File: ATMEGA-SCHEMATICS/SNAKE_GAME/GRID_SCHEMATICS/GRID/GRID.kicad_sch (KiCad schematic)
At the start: 400 parts, among them J1 Conn_01x04_Pin, J2 Conn_01x04_Pin

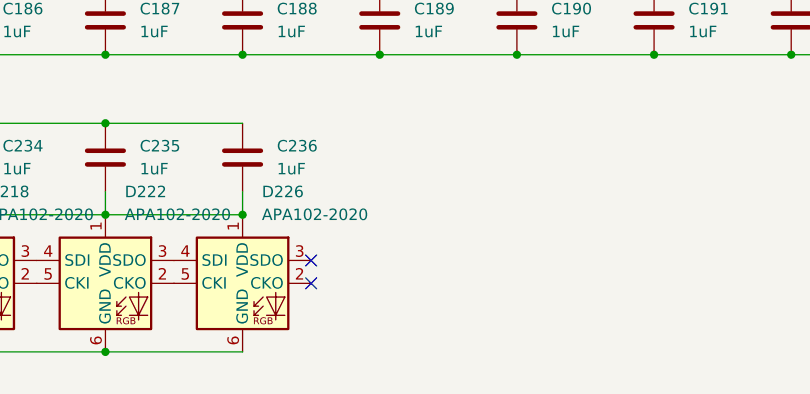
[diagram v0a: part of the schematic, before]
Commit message: .
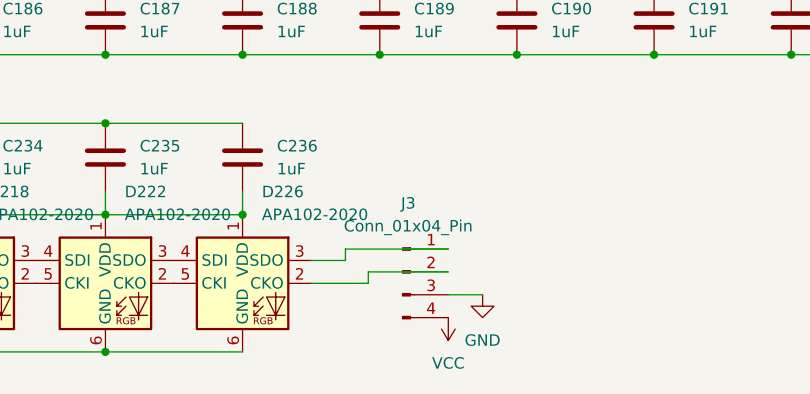
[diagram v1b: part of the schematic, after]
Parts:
- added J3: Conn_01x04_Pin, Connector_PinHeader_2.54mm:PinHeader_1x04_P2.54mm_Vertical, symbol Connector:Conn_01x04_Pin
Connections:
- net GND: now also J3.3 (Pin_3)
- net VCC: now also J3.4 (Pin_4)
- net at D226.2 (CKO): now also J3.2 (Pin_2)
- net at D226.3 (SDO): now also J3.1 (Pin_1)
- no-connect marks 2 -> 0

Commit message: .
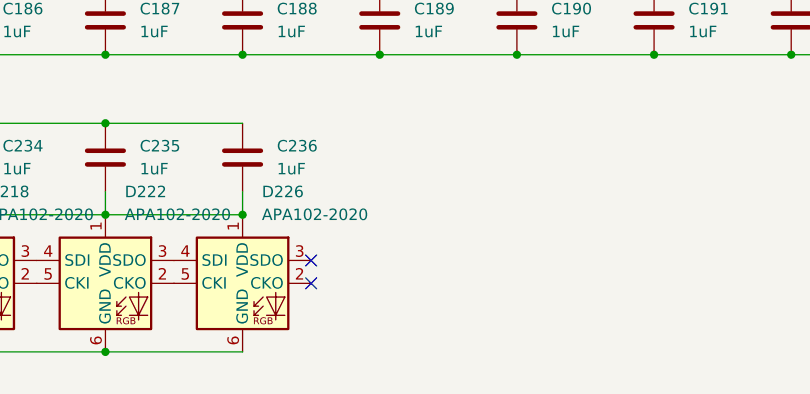
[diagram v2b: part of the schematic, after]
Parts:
- removed J3: Conn_01x04_Pin, Connector_PinHeader_2.54mm:PinHeader_1x04_P2.54mm_Vertical, symbol Connector:Conn_01x04_Pin
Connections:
- no-connect marks 0 -> 2
